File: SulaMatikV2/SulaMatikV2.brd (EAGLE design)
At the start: 66 x 61 mm, 39 parts, among them IC1 REG1117, Q1 2N3904, Q2 2N5551, Q3 2N5551

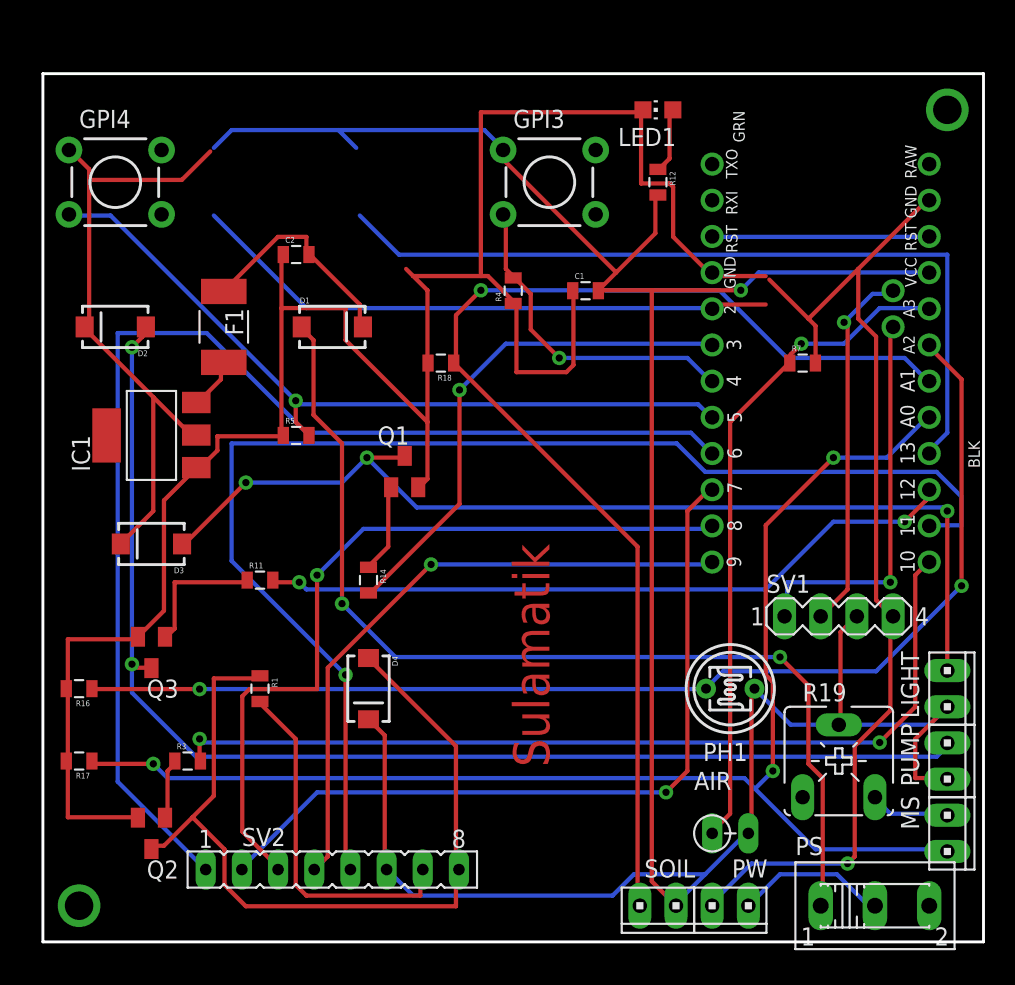
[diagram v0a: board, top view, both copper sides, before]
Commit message: v2
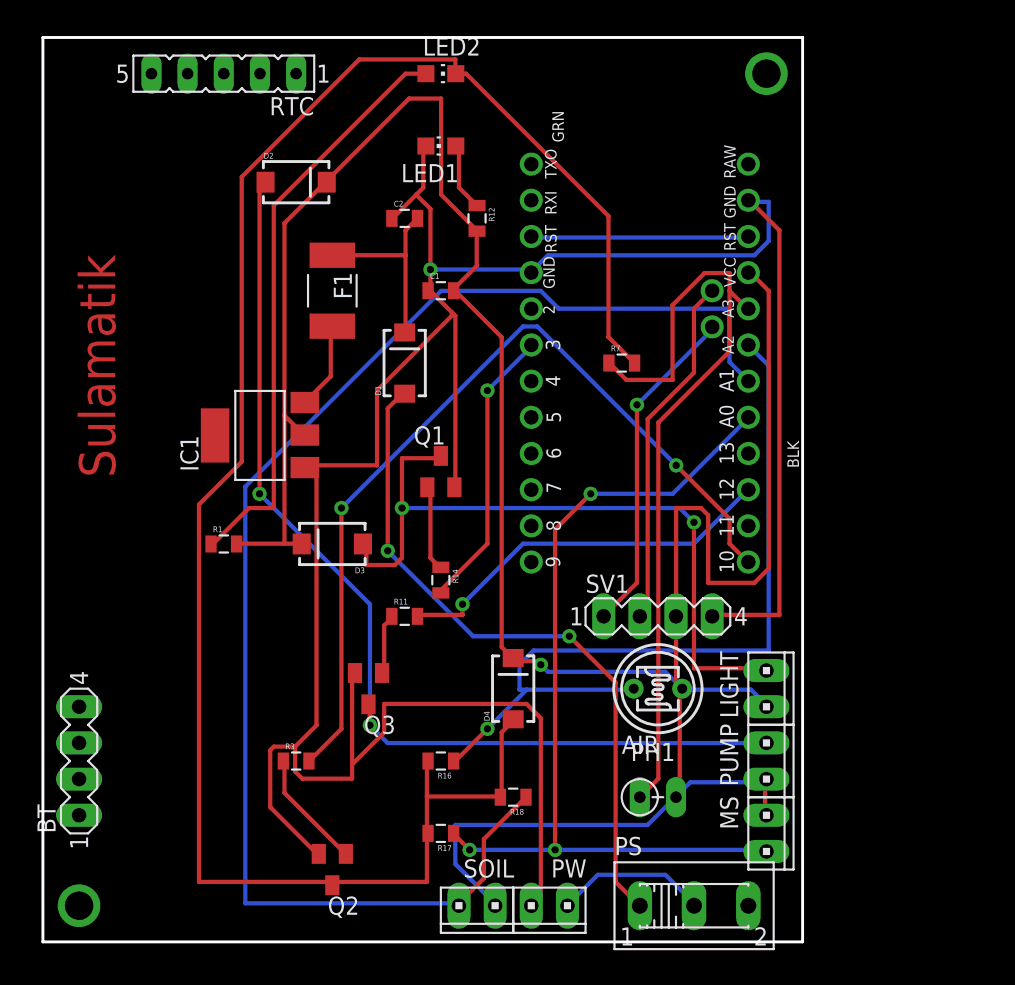
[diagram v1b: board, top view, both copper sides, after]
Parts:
- removed GPI3, GPI4: SWITCH-MOMENTARY-2PTH, SparkFun-Electromechanical:TACTILE-PTH
- removed R19: 10K, pot:CA6V
- removed R4, R5: 10k, SparkFun-Passives:0805
- removed SV2: (no value), con-lsta:FE08
- added BT: (no value), con-lstb:MA04-1
- added LED2: (no value), led:CHIP-LED0805
- added RTC: (no value), con-lsta:FE05-1
- moved R18 30.9 mm to (35.6, 12.7)
- moved R16 25.9 mm to (30.5, 15.2)
- moved R17 25.9 mm to (30.5, 10.2)
- moved D2 16.3 mm to (20.3, 55.9), turned to 0 degrees
- moved LED1 15.5 mm to (30.5, 58.4)
- moved Q3 15.5 mm to (25.4, 20.3)
- moved Q2 13.0 mm to (22.9, 7.62)
- moved R12 13.0 mm to (33.0, 53.3)
- moved JP7 12.7 mm to (36.8, 29.2)
- moved LIGHT 12.7 mm to (53.3, 20.3)
- moved MS 12.7 mm to (53.3, 10.2)
- moved PS 12.7 mm to (48.3, 5.08)
- moved PUMP 12.7 mm to (53.3, 15.2)
- moved R7 12.7 mm to (43.2, 43.2)
- moved SV1 12.7 mm to (45.7, 25.4)
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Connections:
- new net N$12: RTC.2
- new net N$14: RTC.1
- new net N$15: BT.4
- new net N$16: BT.3
- new net N$21: BT.1
- new net N$22: LED2.A, R1.1
- new net N$8: RTC.4
- new net SGND: D4.A, LED2.C, Q2.3, R16.2, R17.2, R18.2, R7.2
- net D4: no longer GPI3.3, R4.2
- net D5: no longer GPI4.3, R5.2
- net D6: no longer SV2.1
- net D7: no longer SV2.2
- net D8: no longer SV2.3
- net D9: no longer SV2.4
- net GND: no longer R16.2, R17.2, R18.2, R4.1, R5.1, R7.2
- net MOSI: no longer SV2.5
- net N$10: now also RTC.3; no longer D4.A, Q2.3, R1.1, SV2.8
- net N$17: now also BT.2; no longer MS.2, R19.E
- net N$3: now also RTC.5; no longer R1.2, SV2.7
- net VCC: now also MS.2, R1.2; no longer GPI3.1, GPI4.1, R19.S, SV2.6
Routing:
- net SGND: track 0.00 -> 132.0 mm
- net MOSI: track 90.5 -> 0.00 mm, vias 1 -> 0
- net D6: track 85.5 -> 0.00 mm
- net N$10: track 60.3 -> 0.00 mm
- net SCK: track 56.9 -> 0.00 mm
- net D8: track 55.8 -> 0.00 mm, vias 1 -> 0
- net D7: track 54.8 -> 0.00 mm, vias 1 -> 0
- net D5: track 53.9 -> 0.00 mm, vias 1 -> 0
- net VCC: track 241.1 -> 192.5 mm
- net D9: track 44.6 -> 0.00 mm, vias 1 -> 0
- net D2: track 41.7 -> 0.00 mm
- net N$22: track 0.00 -> 41.2 mm
- net GND: track 226.2 -> 185.3 mm
- net A0: track 96.7 -> 61.9 mm
- net A2: track 81.9 -> 57.0 mm, vias 2 -> 1
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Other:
- board size 66 x 61 mm -> 53.3 x 63.5 mm
